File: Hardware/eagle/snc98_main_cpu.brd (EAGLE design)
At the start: 168.2 x 30 mm, 89 parts, among them IC1 MCP170333MB, M1 IRLML2244, M12 IRLML2244, M2 IRLML2244, M3 IRLML2244, T1 BCR135, T2 BCR135, T3 BCR185, U1 74HC4051_MUX, U2 DS18B20, U3 ATMEGA1284P-PU, U4 TLV70033 / TC1185, Y2 12MHz

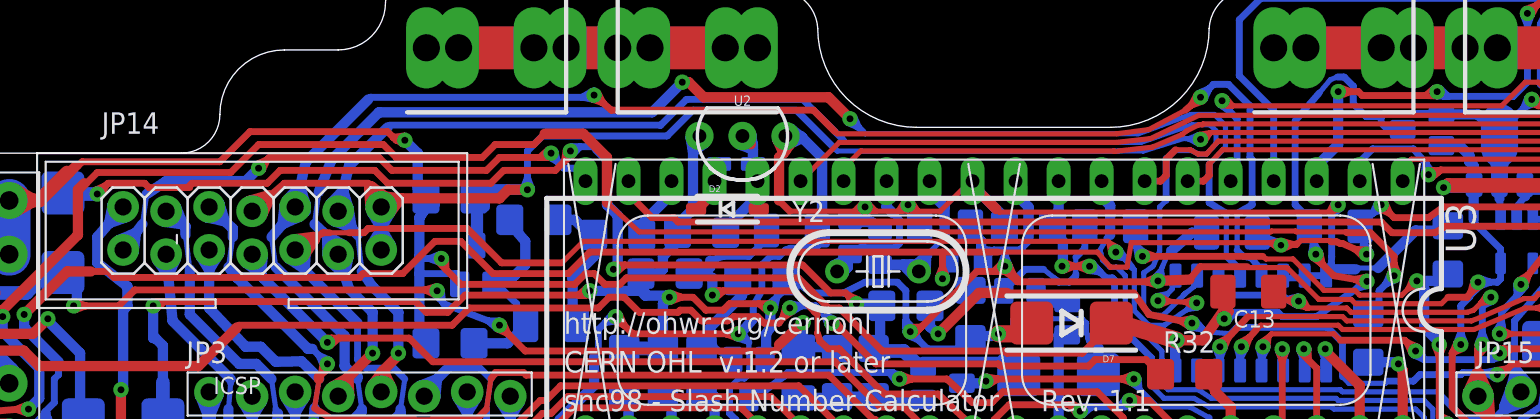
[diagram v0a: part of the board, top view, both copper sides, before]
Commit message: Gerber file added
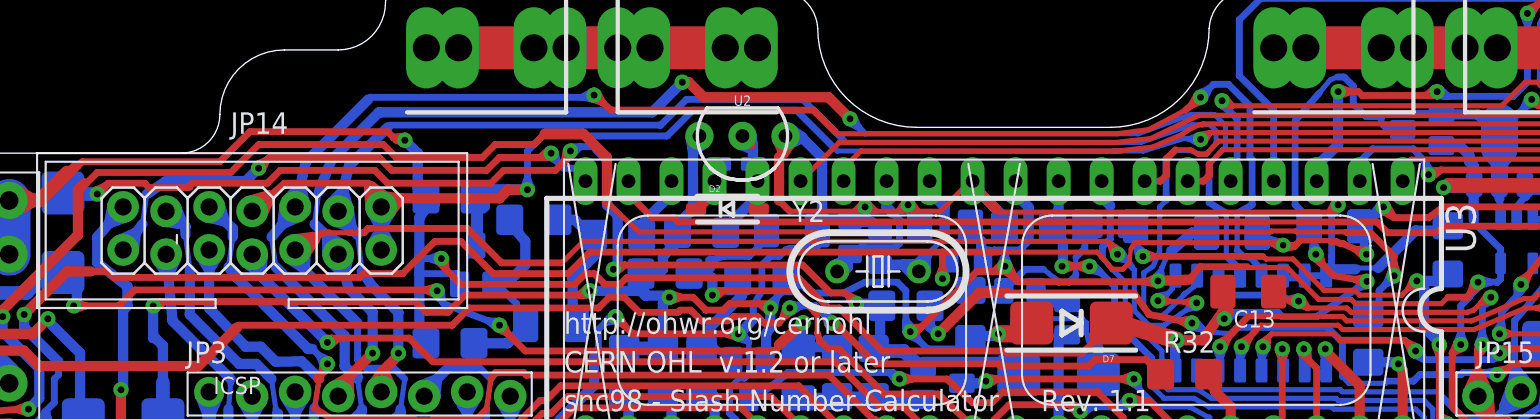
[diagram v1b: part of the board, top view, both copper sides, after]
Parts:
- added C17, C19: 1µ, rcl:C1206K
- added C23: 220n, SparkFun:0805
- C20, C21: value 4.7uF -> 1uF
- C7, C8: value 15pF -> 22pF
- R25: value 100 -> 47
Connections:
- net DTR: now also C23.4
- net GND: now also C17.2, C19.2
- net R_: now also C23.3
- net VCC: now also C17.1
- net V_IN: now also C19.1
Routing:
- net GND: track 214.0 -> 215.9 mm
- net DTR: track 102.4 -> 103.0 mm
- net R_: track 10.3 -> 10.8 mm
